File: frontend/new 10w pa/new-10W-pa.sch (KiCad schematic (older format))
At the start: 43 parts, among them CN1 BREAKOUT, K1 D3002, P1 CONN_01X02, P2 CONN_02X01, P3 External 12V-13.8V (OSTTC0221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, P4 CONN_01X02, P5 CONN_01X02, Q1 FDV301, Q2 FDV301, Q3 RD16HHF1, T1 TRANSFO, T2 OUT_TRANSF, U1 4050, U6 LP2951-50D, U7 LP2951-50D

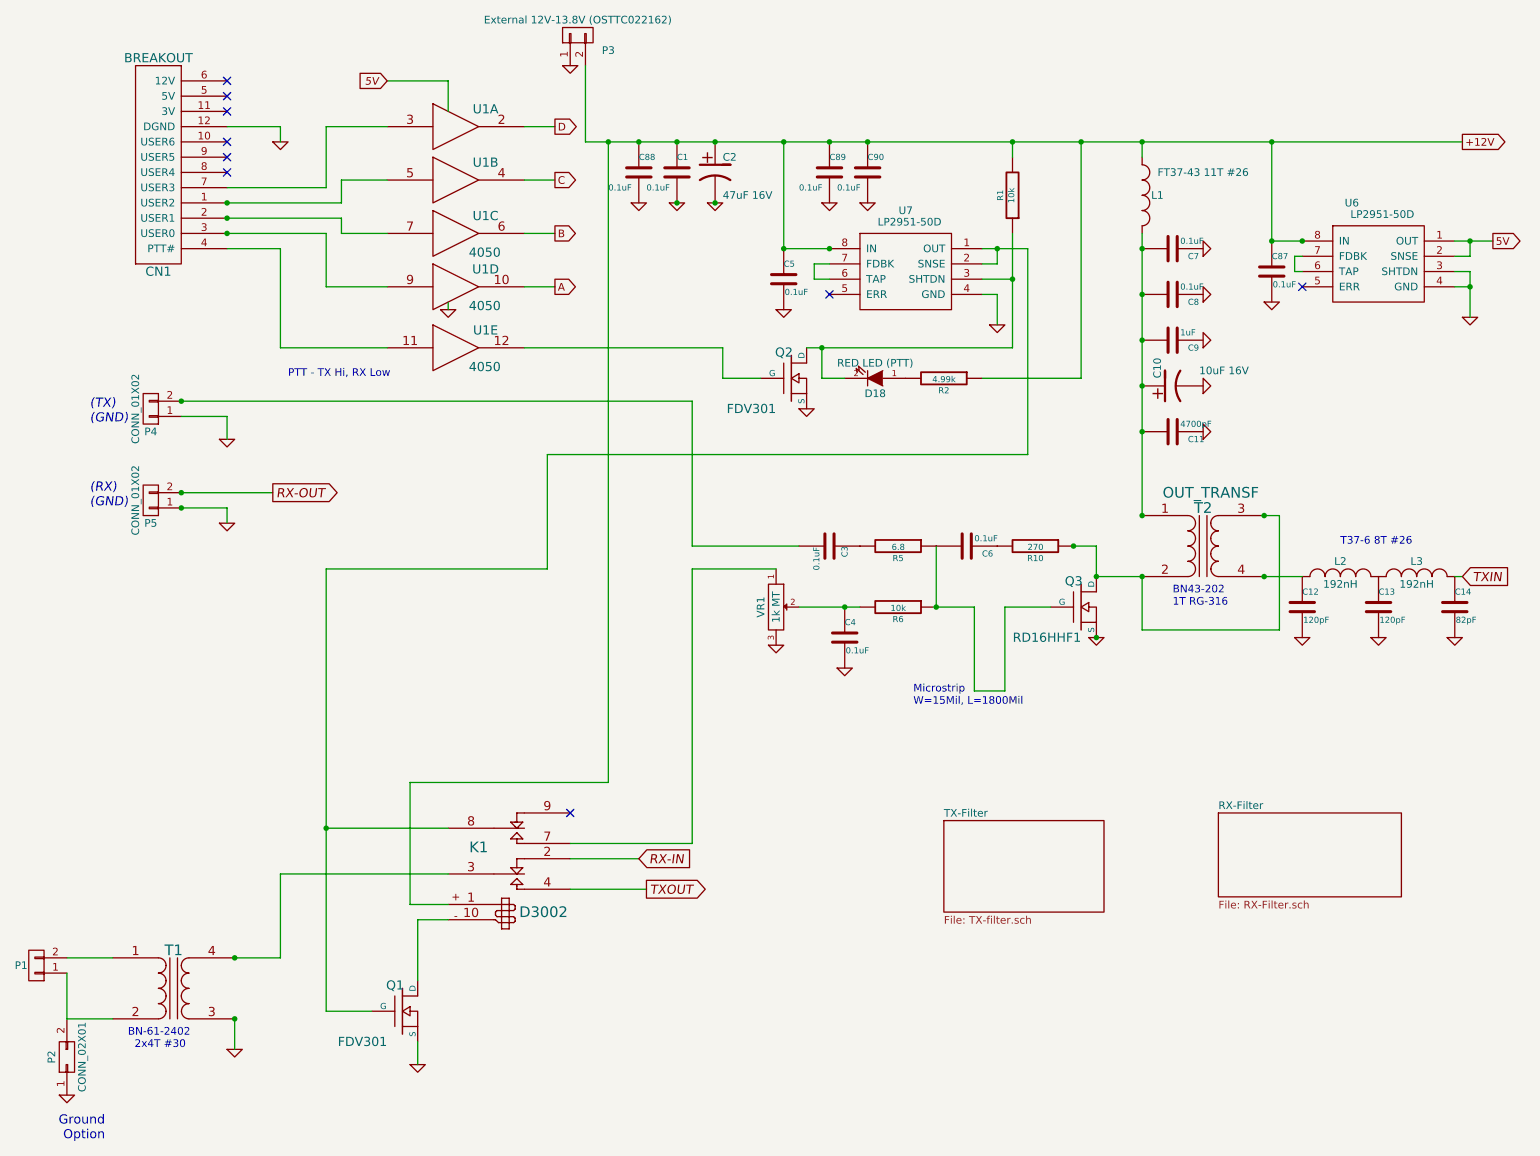
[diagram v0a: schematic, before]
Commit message: first pass for Oshpark
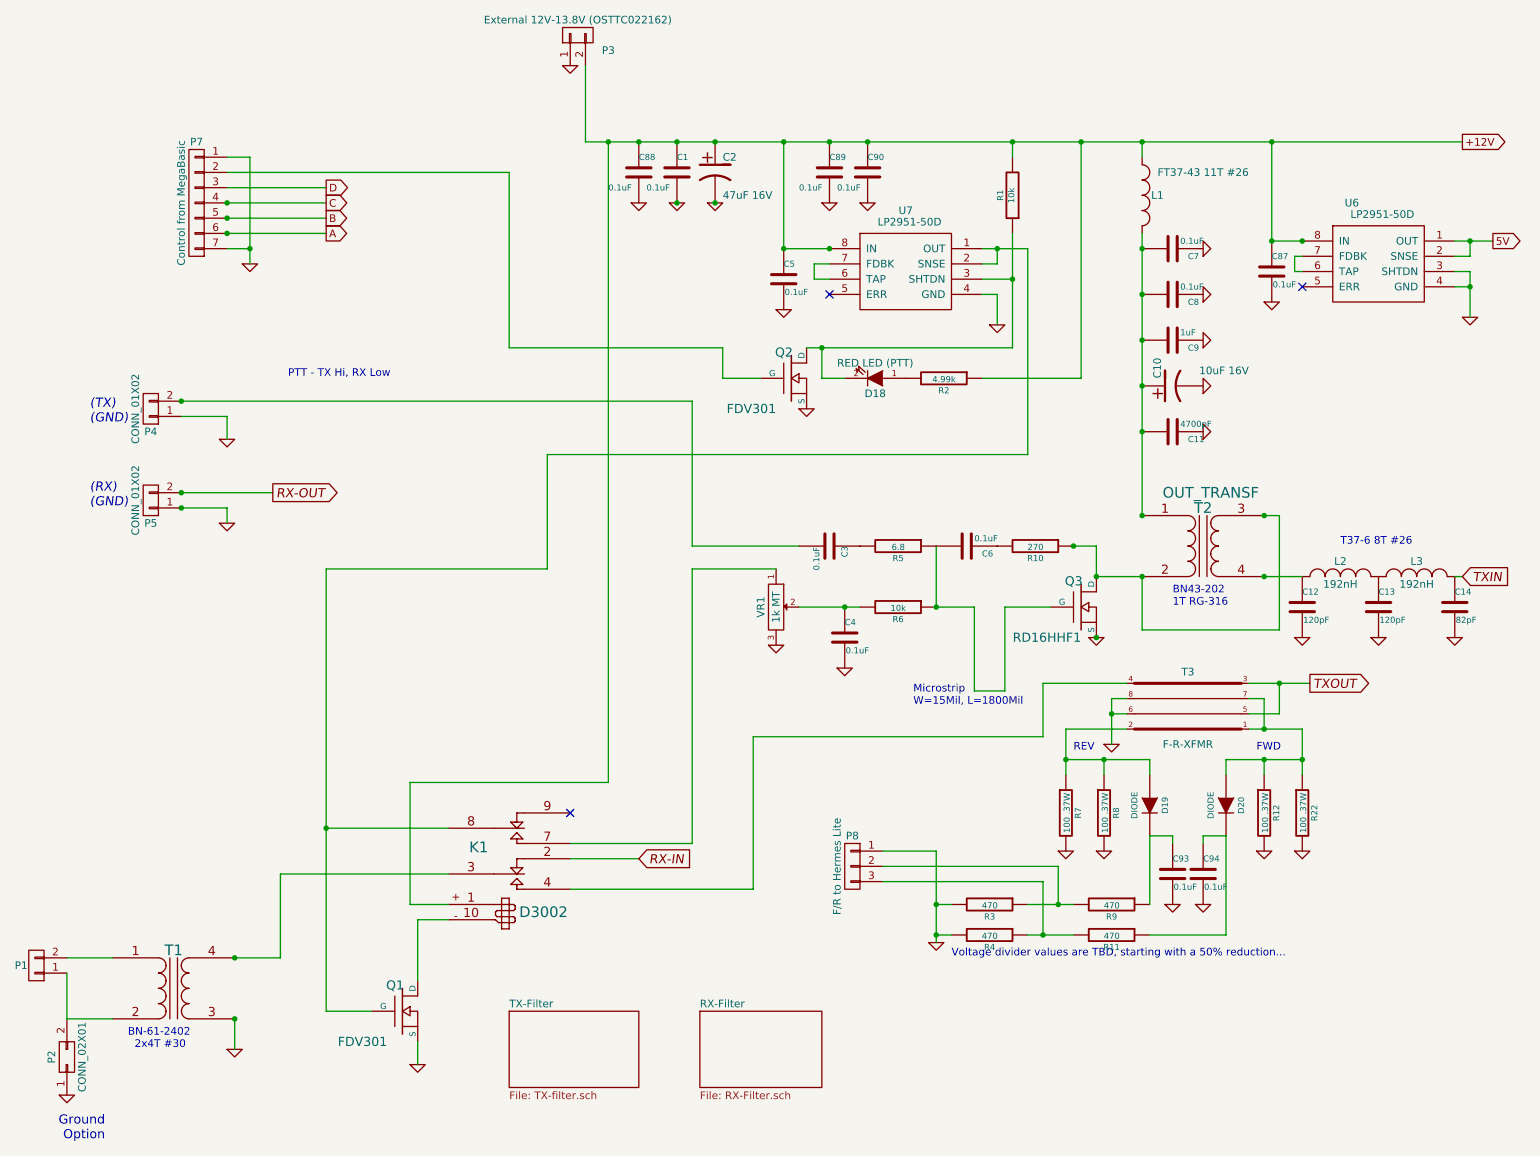
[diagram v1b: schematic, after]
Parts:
- removed CN1: BREAKOUT, HERMESLITE:BREAKOUT, symbol BREAKOUT
- removed U1: 4050, Housings_SOIC:SOIC-16_3.9x9.9mm_Pitch1.27mm, symbol 4050
- added C93, C94: 0.1uF, HERMESLITE:C_0805, symbol C
- added D19, D20: DIODE, Diodes_SMD:Diode-SMA_Standard, symbol DIODE
- added P7: Control from MegaBasic, Pin_Headers:Pin_Header_Straight_1x07, symbol CONN_01X07
- added P8: F/R to Hermes Lite, Pin_Headers:Pin_Header_Straight_1x03, symbol CONN_01X03
- added R11, R3, R4, R9: 470, HERMESLITE:R_0805, symbol R
- added R12, R22, R7, R8: 100 .37W, HERMESLITE:R_0805, symbol R
- added T3: F-R-XFMR, HERMESLITE:F_R_Transf, symbol F-R-XFMR
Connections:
- net A: now also P7.6 (P6)
- net B: now also P7.5 (P5)
- net C: now also P7.4 (P4)
- net D: now also P7.3 (P3)
- net GND: now also C93.2, C94.2, P7.1 (P1), P7.7 (P7), P8.1 (P1), R12.2, R22.2, R3.2, R4.2, R7.2, R8.2, T3.6, T3.8
- net TXOUT: now also T3.3, T3.5; no longer K1.4 (T1)
- net at Q2.G: now also P7.2 (P2)
- net VCC renamed 5V
- new net: K1.4 (T1), T3.4
- new net: D20.1 (A), R12.1, R22.1, T3.1, T3.7
- new net: D19.1 (A), R7.1, R8.1, T3.2
- new net: C94.1, D20.2 (K), R11.1
- new net: P8.3 (P3), R11.2, R4.1
- new net: C93.1, D19.2 (K), R9.1
- new net: P8.2 (P2), R3.1, R9.2
- no-connect marks 9 -> 3
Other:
- note added: "FWD"
- note added: "REV"
- note added: "Voltage divider values are TBD, starting with a 50% reduction..."
